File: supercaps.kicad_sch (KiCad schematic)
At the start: 11 parts, among them J7 XT30_F, J8 XT30_F, U5 OPA551U

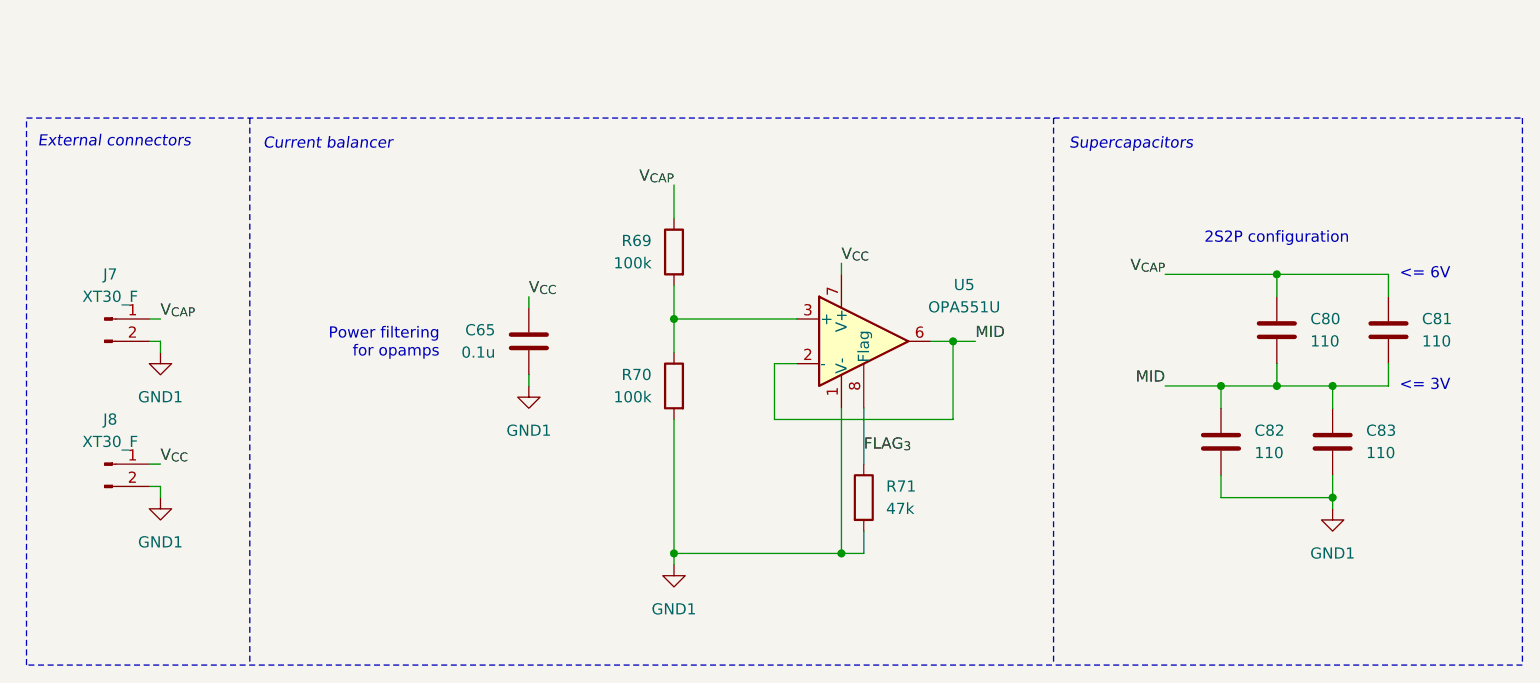
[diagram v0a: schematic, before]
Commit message: Finalize balancing circuit
Looks pretty stable to me
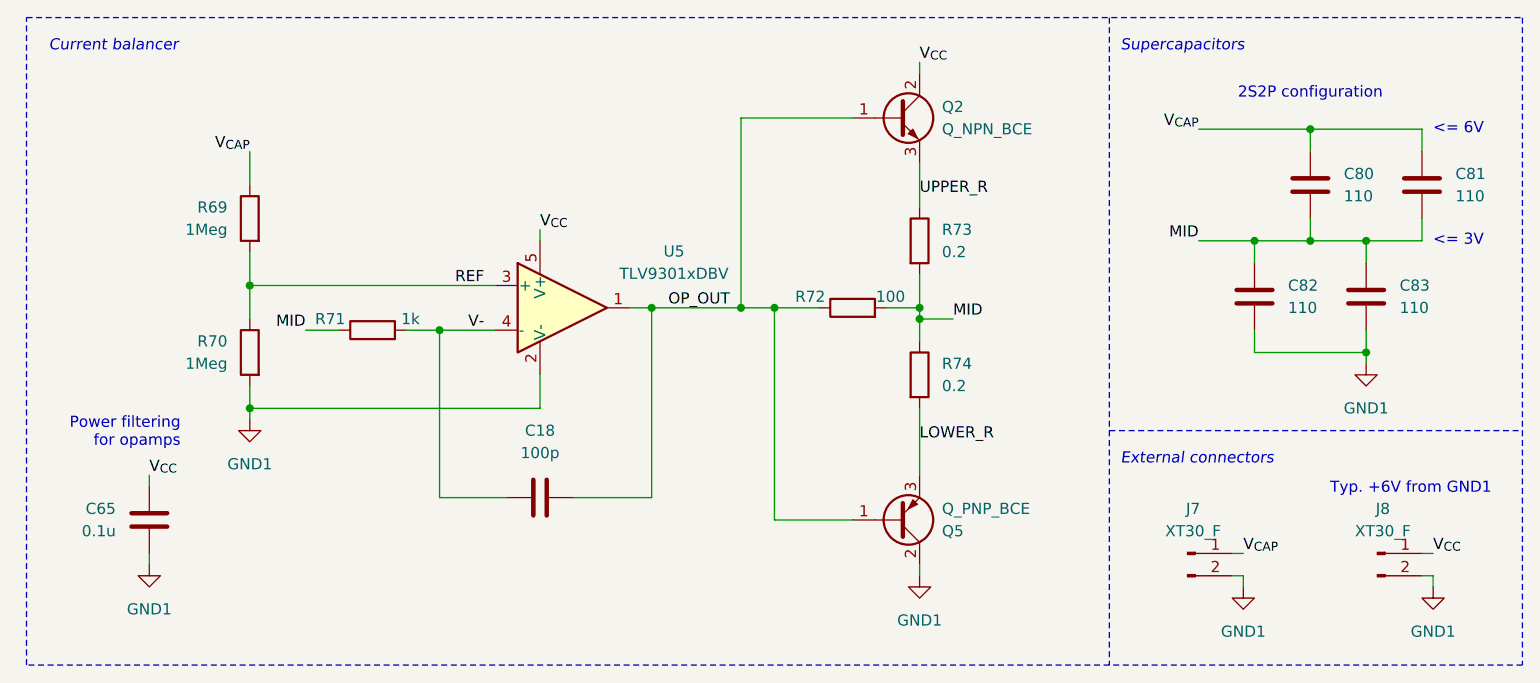
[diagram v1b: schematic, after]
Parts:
- removed U5: OPA551U, Package_SO:SOIC-8_3.9x4.9mm_P1.27mm, symbol Amplifier_Operational:OPA551U
- added C18: 100p, Capacitor_SMD:C_0603_1608Metric_Pad1.08x0.95mm_HandSolder, symbol Device:C
- added Q2: Q_NPN_BCE, symbol Transistor_BJT:Q_NPN_BCE
- added Q5: Q_PNP_BCE, symbol Transistor_BJT:Q_PNP_BCE
- added R72: 100, Resistor_SMD:R_0603_1608Metric_Pad0.98x0.95mm_HandSolder, symbol Device:R
- added R73, R74: 0.2, Resistor_SMD:R_0603_1608Metric_Pad0.98x0.95mm_HandSolder, symbol Device:R
- added U5: TLV9301xDBV, Package_TO_SOT_SMD:SOT-23-5_HandSoldering, symbol Amplifier_Operational:TLV9301xDBV
- R69, R70: value 100k -> 1Meg
- R71: value 47k -> 1k
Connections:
- net FLAG_{3} is gone; now on net MID: R71.1
- net GND1: now also Q5.2 (C), U5.2 (V-); no longer R71.2
- net MID: now also R72.2, R73.2, R74.1
- net V_{CC}: now also Q2.2 (C), U5.5 (V+)
- net REF: now reaches R69.2, R70.1
- net REF: now also U5.3 (+)
- new net LOWER_R: Q5.3 (E), R74.2
- new net OP_OUT: C18.2, Q2.1 (B), Q5.1 (B), R72.1, U5.1
- new net UPPER_R: Q2.3 (E), R73.1
- new net V-: C18.1, R71.2, U5.4 (-)
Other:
- note added: "Typ. +6V from GND1"
- moved on the sheet: C65, C80, C81, C82, C83, J7, J8, R69, R70
